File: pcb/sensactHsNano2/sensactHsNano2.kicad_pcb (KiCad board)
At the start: 2 copper layers, 90 x 61.5 mm, 144 parts, among them J1 PROG, J2 SensactBusConnector, J3 CAN+24V, J4 HR911105A, J5 Audio, J6 Conn_01x03, J7 USB_C_Receptacle_USB2.0, J8 Conn_01x10, Q1 BC817, Q2 BC817, SW1 TERM ON, SW2 Prog, SW3 Reset, SW4 PROG_PWR, U1 TAS5805M, U10 ADS1115IDGS, U11 L78L15_SOT89, U12 SRV05, U2 LAN8720A, U3 ESP32, U4 DS2482, U5 SN65HVD230, U6 CH340K, U7 MP4420, U8 LM358, U9 MCP4728, X1 50MHz

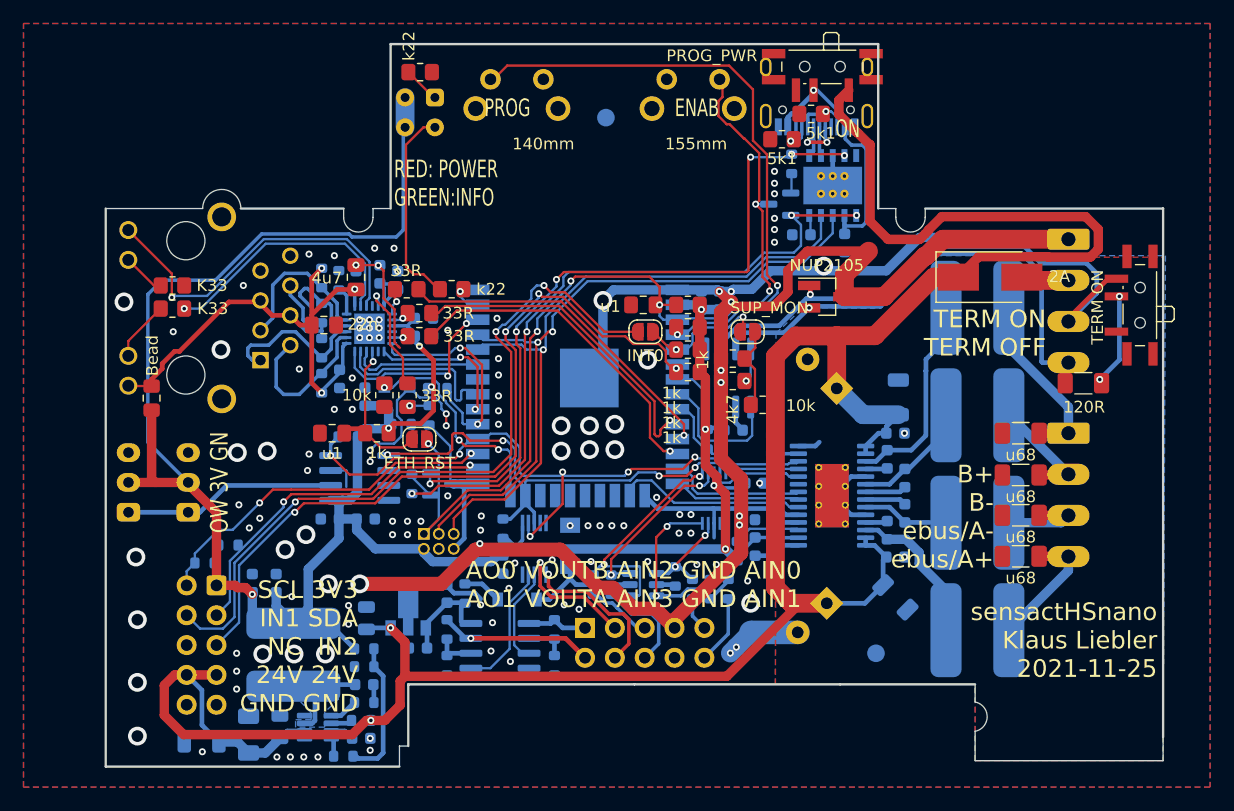
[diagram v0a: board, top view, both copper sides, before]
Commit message: Sicherung
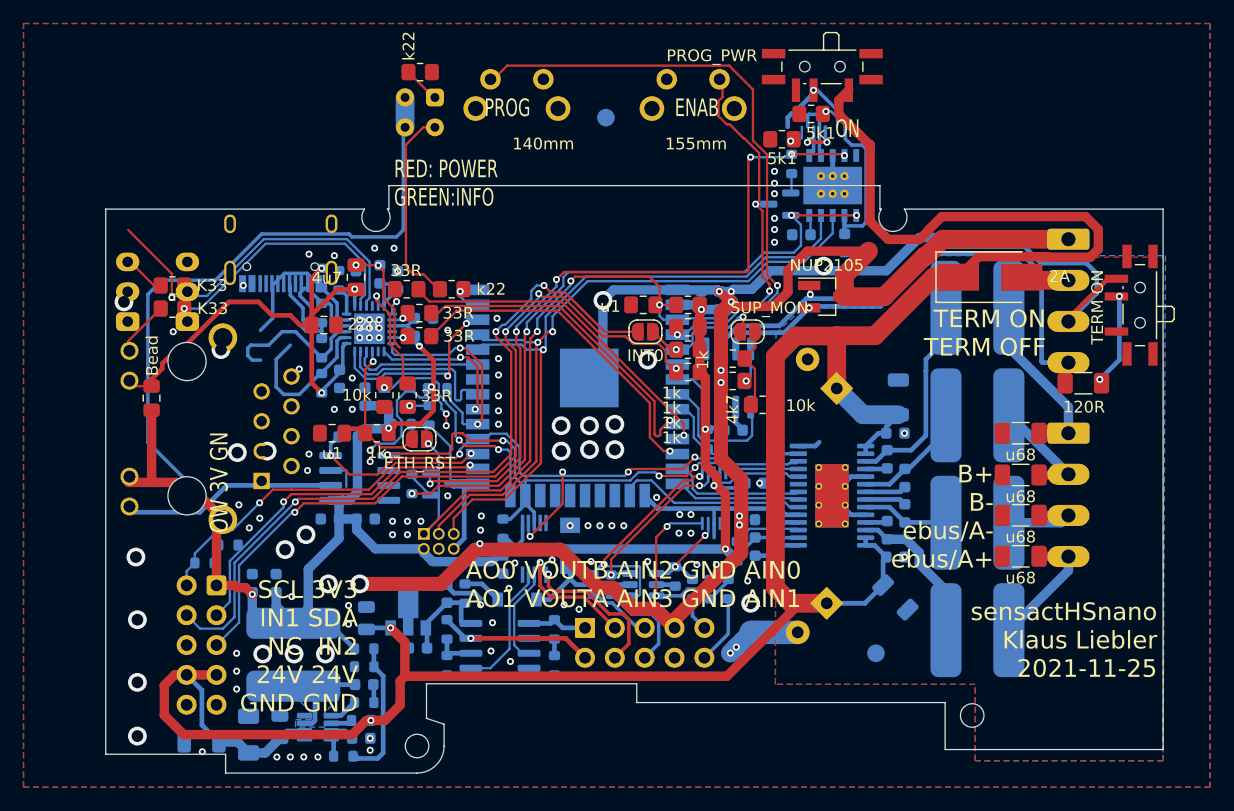
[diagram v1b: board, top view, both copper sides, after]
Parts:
- moved J7 47.5 mm to (119.9, 110.1)
- moved J6 16.2 mm to (112.0, 117.4)
- moved J4 10.3 mm to (111.9, 126.5)
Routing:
- net GND: vias 125 -> 122
- net /eth/VDD2A: vias 3 -> 4
- net /eth/RX_P: vias 0 -> 1
- net +3V3: vias 8 -> 9
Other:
- board size 90 x 61.5 mm -> 90 x 50 mm
